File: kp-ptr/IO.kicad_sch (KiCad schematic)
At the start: 25 parts, among them J6 Conn_01x06_Male, J7 Conn_01x10_Male, J8 Conn_01x06_Male, J9 Conn_01x02_Male, Q1 NMOS_SOT23

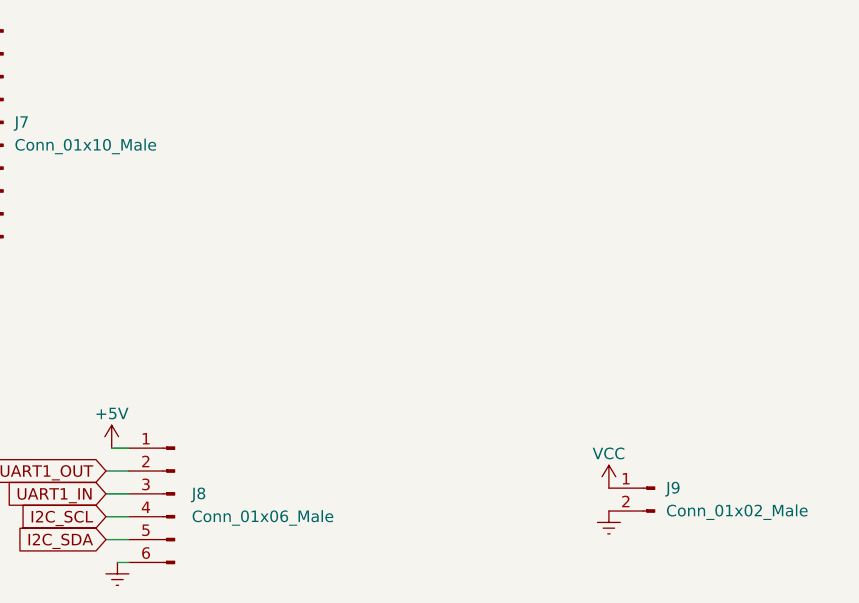
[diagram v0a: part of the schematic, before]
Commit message: PCB update
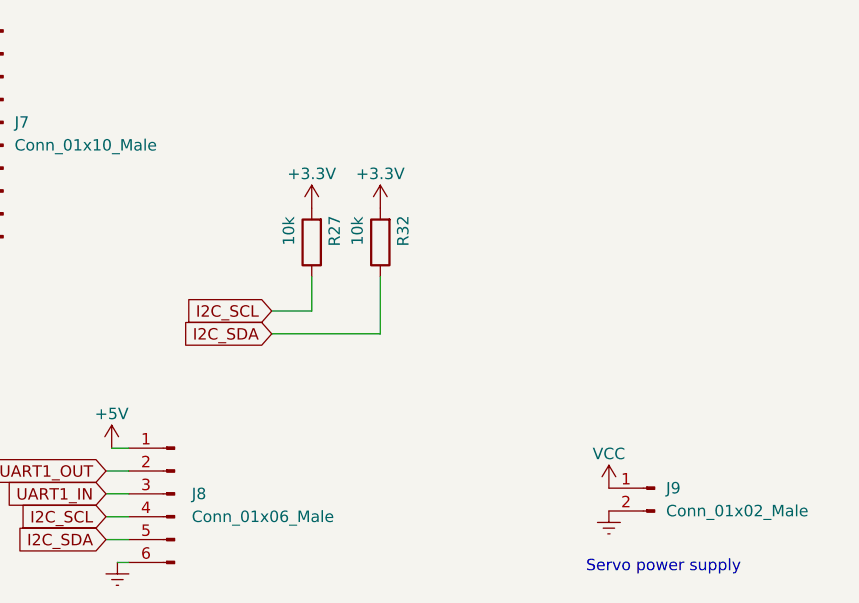
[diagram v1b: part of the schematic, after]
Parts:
- added R27, R32: 10k, Resistor_SMD:R_0402_1005Metric, symbol Device:R
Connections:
- net +3V3: now also R27.2, R32.2
- net I2C_SCL: now also R27.1
- net I2C_SDA: now also R32.1
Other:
- note added: "Servo power supply"
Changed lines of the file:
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@@
+    (stroke (width 0) (type default) (color 0 0 0 0))
+  )
+  (wire (pts (xy 105.41 158.75) (xy 105.41 162.56))
     (stroke (width 0) (type default) (color 0 0 0 0))
   )
@@
     (stroke (width 0) (type default) (color 0 0 0 0))
   )
+  (wire (pts (xy 100.965 165.1) (xy 113.03 165.1))
+    (stroke (width 0) (type default) (color 0 0 0 0))
+  )
   (wire (pts (xy 52.705 144.145) (xy 66.04 144.145))
     (stroke (width 0) (type default) (color 0 0 0 0))
@@
     (stroke (width 0) (type default) (color 0 0 0 0))
   )
+  (wire (pts (xy 105.41 162.56) (xy 100.965 162.56))
+    (stroke (width 0) (type default) (color 0 0 0 0))
+  )
   (wire (pts (xy 59.69 151.765) (xy 59.69 149.225))
     (stroke (width 0) (type default) (color 0 0 0 0))
@@
     (stroke (width 0) (type default) (color 0 0 0 0))
   )
+  (wire (pts (xy 113.03 165.1) (xy 113.03 158.75))
+    (stroke (width 0) (type default) (color 0 0 0 0))
+  )
+  (text "Servo power supply" (at 135.89 191.77 0)
+    (effects (font (size 1.27 1.27)) (justify left bottom))
+  )
   (global_label "UART1_OUT" (shape input) (at 82.55 180.34 180) (fields_autoplaced)
     (effects (font (size 1.27 1.27)) (justify right))
@@
     )
   )
+  (global_label "I2C_SCL" (shape input) (at 100.965 162.56 180) (fields_autoplaced)
+    (effects (font (size 1.27 1.27)) (justify right))
+    (property "Intersheet References" "${INTERSHEET_REFS}" (id 0) (at 90.9924 162.4806 0)
+      (effects (font (size 1.27 1.27)) (justify right) hide)
+    )
+  )
   (global_label "SERVO_2" (shape input) (at 36.83 141.605 180) (fields_autoplaced)
     (effects (font (size 1.27 1.27)) (justify right))
@@
     (effects (font (size 1.27 1.27)) (justify right))
     (property "Intersheet References" "${INTERSHEET_REFS}" (id 0) (at 24.9221 149.1456 0)
+      (effects (font (size 1.27 1.27)) (justify right) hide)
+    )
+  )
+  (global_label "I2C_SDA" (shape input) (at 100.965 165.1 180) (fields_autoplaced)
+    (effects (font (size 1.27 1.27)) (justify right))
+    (property "Intersheet References" "${INTERSHEET_REFS}" (id 0) (at 90.9319 165.0206 0)
       (effects (font (size 1.27 1.27)) (justify right) hide)
     )
@@
     (property "PRICE" "None" (id 9) (at 55.88 95.25 0)
       (effects (font (size 1.27 1.27)) (justify left bottom) hide)
+    )
+    (pin "1")
+    (pin "2")
+  )
+  (symbol (lib_id "Device:R") (at 105.41 154.94 180) (unit 1)
+    (in_bom yes) (on_board yes)
+    (property "Reference" "R27" (id 0) (at 107.95 153.67 90))
+    (property "Value" "10k" (id 1) (at 102.87 153.67 90))
+    (property "Footprint" "Resistor_SMD:R_0402_1005Metric" (id 2) (at 107.188 154.94 90)
+      (effects (font (size 1.27 1.27)) hide)
+    )
+    (property "Datasheet" "~" (id 3) (at 105.41 154.94 0)
+      (effects (font (size 1.27 1.27)) hide)
     )
     (pin "1")
@@
     (pin "2")
   )
+  (symbol (lib_id "Device:R") (at 113.03 154.94 180) (unit 1)
+    (in_bom yes) (on_board yes)
+    (property "Reference" "R32" (id 0) (at 115.57 153.67 90))
+    (property "Value" "10k" (id 1) (at 110.49 153.67 90))
+    (property "Footprint" "Resistor_SMD:R_0402_1005Metric" (id 2) (at 114.808 154.94 90)
+      (effects (font (size 1.27 1.27)) hide)
+    )
+    (property "Datasheet" "~" (id 3) (at 113.03 154.94 0)
+      (effects (font (size 1.27 1.27)) hide)
+    )
+    (pin "1")
+    (pin "2")
+  )
   (symbol (lib_id "Device:R") (at 48.895 146.685 270) (unit 1)
     (in_bom yes) (on_board yes)
@@
     (pin "1")
     (pin "2")
+  )
+  (symbol (lib_id "power:+3.3V") (at 113.03 151.13 0) (unit 1)
+    (in_bom yes) (on_board yes)
+    (property "Reference" "#PWR0176" (id 0) (at 113.03 154.94 0)
+      (effects (font (size 1.27 1.27)) hide)
+    )
+    (property "Value" "+3.3V" (id 1) (at 113.03 147.32 0))
+    (property "Footprint" "" (id 2) (at 113.03 151.13 0)
+      (effects (font (size 1.27 1.27)) hide)
+    )
+    (property "Datasheet" "" (id 3) (at 113.03 151.13 0)
+      (effects (font (size 1.27 1.27)) hide)
+    )
+    (pin "1")
   )
   (symbol (lib_id "power:Earth") (at 133.35 57.15 0) (unit 1)
@@
       (effects (font (size 1.27 1.27)) hide)
     )
+    (pin "1")
+  )
+  (symbol (lib_id "power:+3.3V") (at 105.41 151.13 0) (unit 1)
+    (in_bom yes) (on_board yes)
+    (property "Reference" "#PWR0133" (id 0) (at 105.41 154.94 0)
+      (effects (font (size 1.27 1.27)) hide)
+    )
+    (property "Value" "+3.3V" (id 1) (at 105.41 147.32 0))
+    (property "Footprint" "" (id 2) (at 105.41 151.13 0)
+      (effects (font (size 1.27 1.27)) hide)
+    )
+    (property "Datasheet" "" (id 3) (at 105.41 151.13 0)
+      (effects (font (size 1.27 1.27)) hide)
+    )
